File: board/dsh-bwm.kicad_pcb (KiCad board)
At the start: 2 copper layers, 136.5 x 78.7 mm, 37 parts, among them IC1 MP4462DN-Z-LF, IC2 MAX485CSA+T, J1 MPM-15-24, J2 Power, J3 Connections, J4 LED, K1 833H-1C-C-24VDC, K2 833H-1C-C-24VDC, K3 833H-1C-C-24VDC, K4 833H-1C-C-24VDC, Q1 IRLB8721PBF, U1 Pico

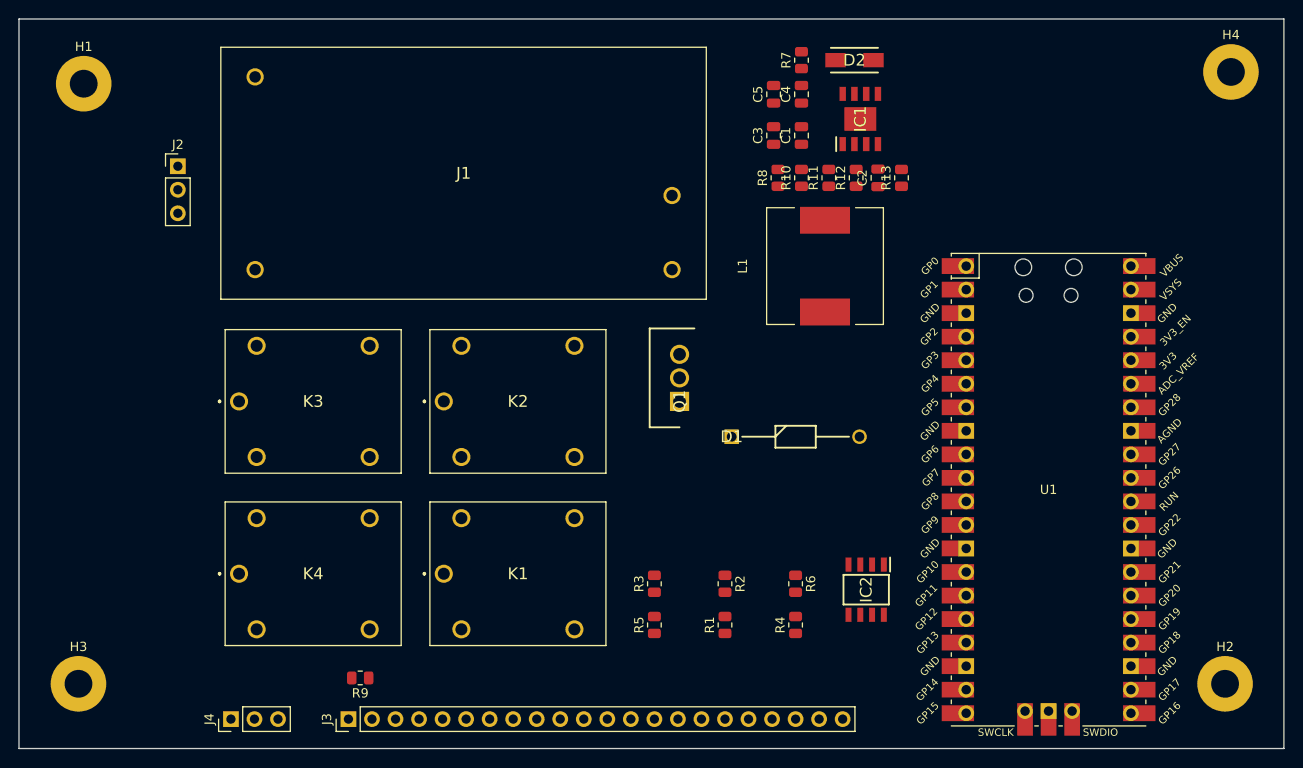
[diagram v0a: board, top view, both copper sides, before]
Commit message: Traces, traces everywhere
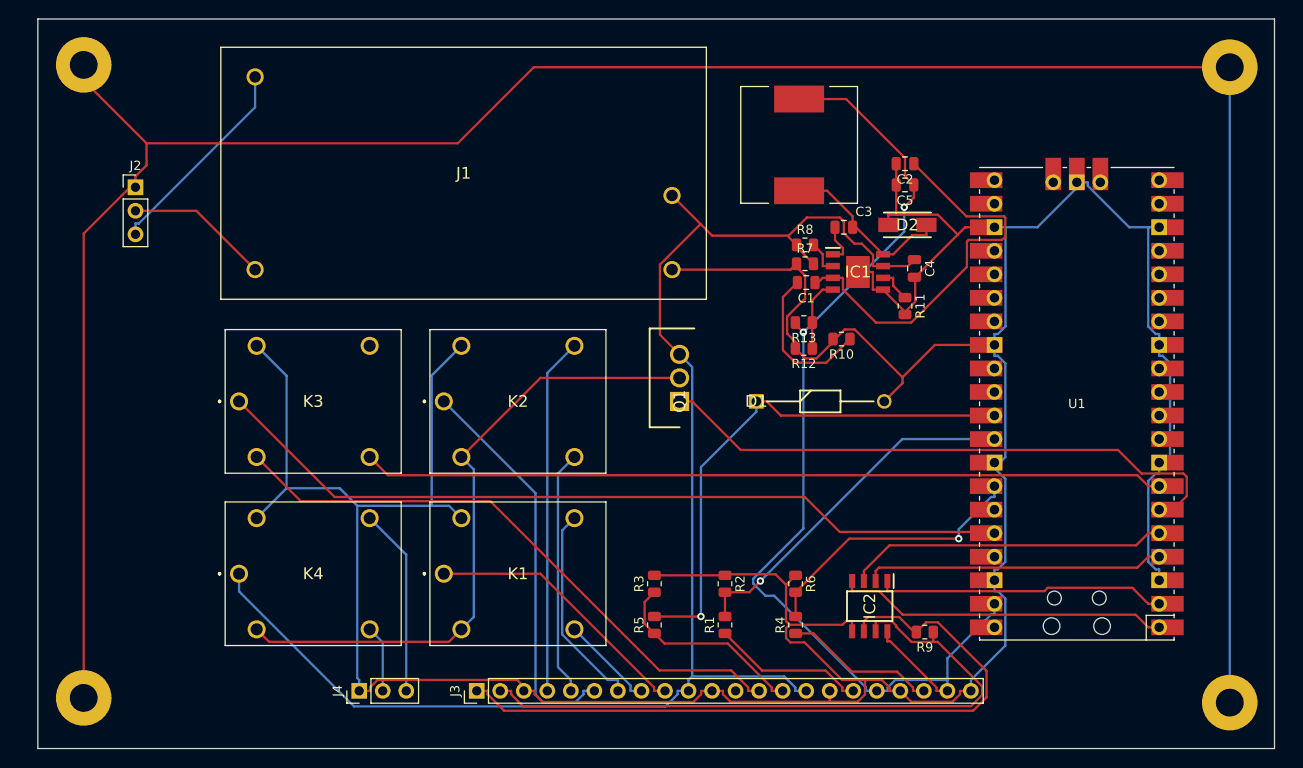
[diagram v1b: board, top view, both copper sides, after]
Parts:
- moved R9 61.1 mm to (187.3, 121.4)
- moved C4 22.4 mm to (186.2, 82.2), turned to -90 degrees
- moved R7 22.0 mm to (174.4, 81.7), turned to 0 degrees
- moved R12 19.3 mm to (174.2, 90.8), turned to 180 degrees
- moved R13 18.8 mm to (174.2, 88.0), turned to 180 degrees
- moved D2 18.7 mm to (185.4, 77.5), turned to 180 degrees
- moved R10 17.9 mm to (178.3, 89.8), turned to 180 degrees
- moved C5 17.2 mm to (185.2, 73.2), turned to 180 degrees
- moved IC1 16.5 mm to (180.1, 82.5), turned to 0 degrees
- moved R11 16.1 mm to (185.2, 86.2), turned to -90 degrees
- moved C1 15.9 mm to (174.5, 83.7), turned to 180 degrees
- moved J4 14.2 mm to (126.3, 127.8)
- moved J3 14.2 mm to (138.9, 127.8)
- moved L1 13.4 mm to (173.7, 68.8)
- moved C3 12.5 mm to (178.6, 77.7), turned to 0 degrees
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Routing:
- net GND: track 0.00 -> 409.3 mm
- net Net-(H1-Pad1): track 0.00 -> 263.4 mm
- net 24V: track 0.00 -> 160.3 mm
- net 5V: track 0.00 -> 117.4 mm, vias 0 -> 2
- net 3v3: track 0.00 -> 87.4 mm
- net ZD: track 0.00 -> 86.5 mm
- net A: track 0.00 -> 77.4 mm
- net B: track 0.00 -> 71.0 mm
- net Net-(K1-Pad2): track 0.00 -> 70.0 mm
- net ZDSENSE: track 0.00 -> 64.9 mm
- net ALARM: track 0.00 -> 63.8 mm
- net COND: track 0.00 -> 57.0 mm, vias 0 -> 1
- net Net-(C1-Pad1): track 0.00 -> 43.3 mm
- net AlarmC2: track 0.00 -> 43.2 mm
- net PSin: track 0.00 -> 38.6 mm, vias 0 -> 1
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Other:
- board size 136.5 x 78.7 mm -> 133.5 x 78.7 mm

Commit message: Bigger is better?
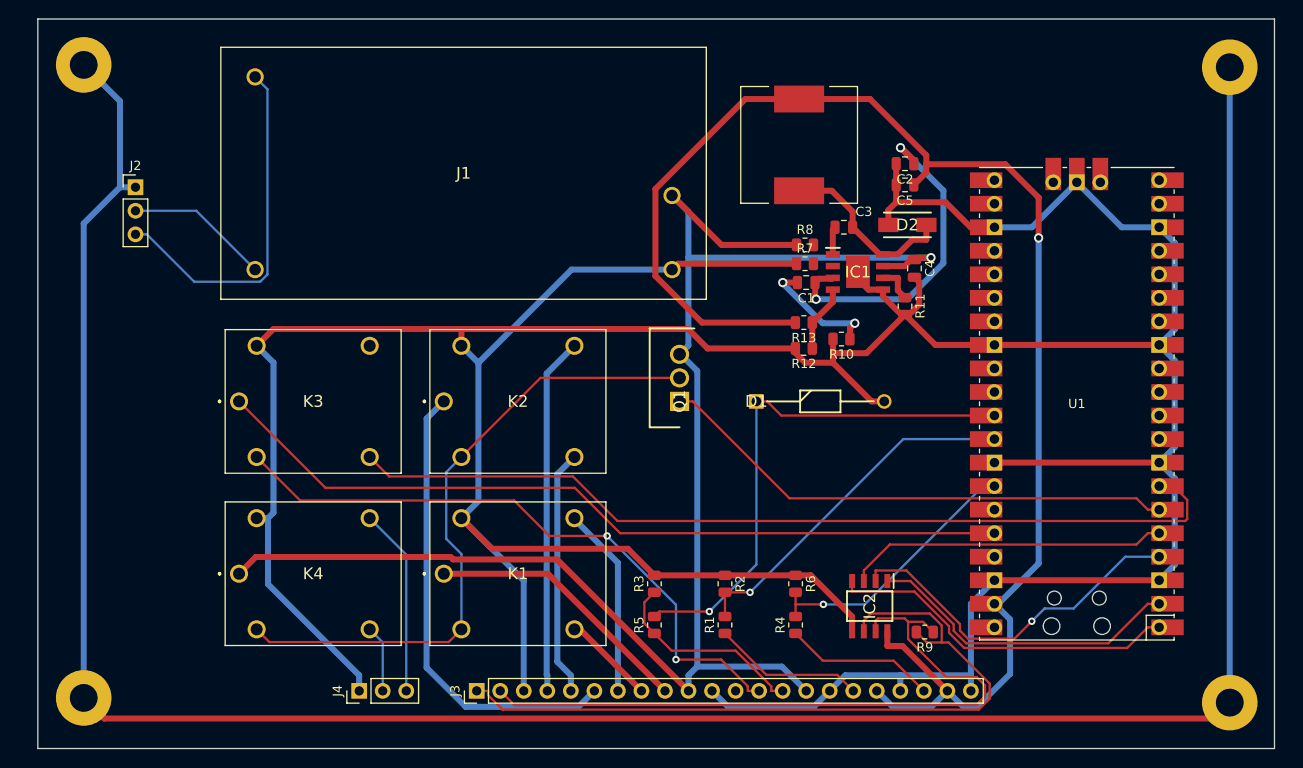
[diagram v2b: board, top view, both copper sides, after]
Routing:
- net GND: track 409.3 -> 462.7 mm
- net 5V: track 117.4 -> 162.0 mm, vias 2 -> 1
- net L1: track 22.6 -> 38.6 mm
- net 24V: track 160.3 -> 171.3 mm, vias 0 -> 1
- net ZD: track 86.5 -> 96.9 mm
- net Net-(C1-Pad1): track 43.3 -> 36.1 mm, vias 0 -> 2
- net ALARM: track 63.8 -> 56.6 mm
- net AlarmC2: track 43.2 -> 50.1 mm
- net RE: track 32.3 -> 38.9 mm, vias 0 -> 1
- net B: track 71.0 -> 74.9 mm
- net Net-(IC1-Pad2): track 3.79 -> 0.00 mm
- net Net-(H1-Pad1): track 263.4 -> 267.2 mm
- net A: track 77.4 -> 81.1 mm
- net Net-(C1-Pad2): track 16.8 -> 13.2 mm, vias 0 -> 2
- net ZDSENSE: track 64.9 -> 68.5 mm, vias 0 -> 2
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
